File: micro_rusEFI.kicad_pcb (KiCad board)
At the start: 2 copper layers, 80.6 x 93.7 mm, 247 parts, among them CN1 100nF, CN2 100nF, CN3 100nF, CN4 100nF, J1 USB_B_Micro, J12 Conn_01x01, J13 Conn_01x01, J14 microSD_HC_Wuerth_693072010801, J15 Conn_01x01, J17 Conn_01x01, J19 Conn_01x06, J2 Conn_02x05_Odd_Even, J3 Conn_01x01, J4 Conn_02x05_Counter_Clockwise, J5 Conn_01x01, J7 TC2030, Q1 IPD30N06S2L-23, SW1 SW_Push, SW2 SW_Push, SW3 SW_Push, SW4 SW_Push, U1 STM32F427VGT6, U10 VNLD5090, U2 TLE8888QK, U3 molex_48pin_MRE, U31 MIC4427, U32 MIC4427, U33 MIC4427, U35 MCP6004, U36 MCP6004, U4 TLE9201SG, U46 MCP6004, U5 LM1117-3.3, U6 W25Q128JVSIQ, U7 XC6206 3.3V, U8 MCP6004, U9 VNLD5090, X1 8MHz 20pF, Y2 32768 Hz

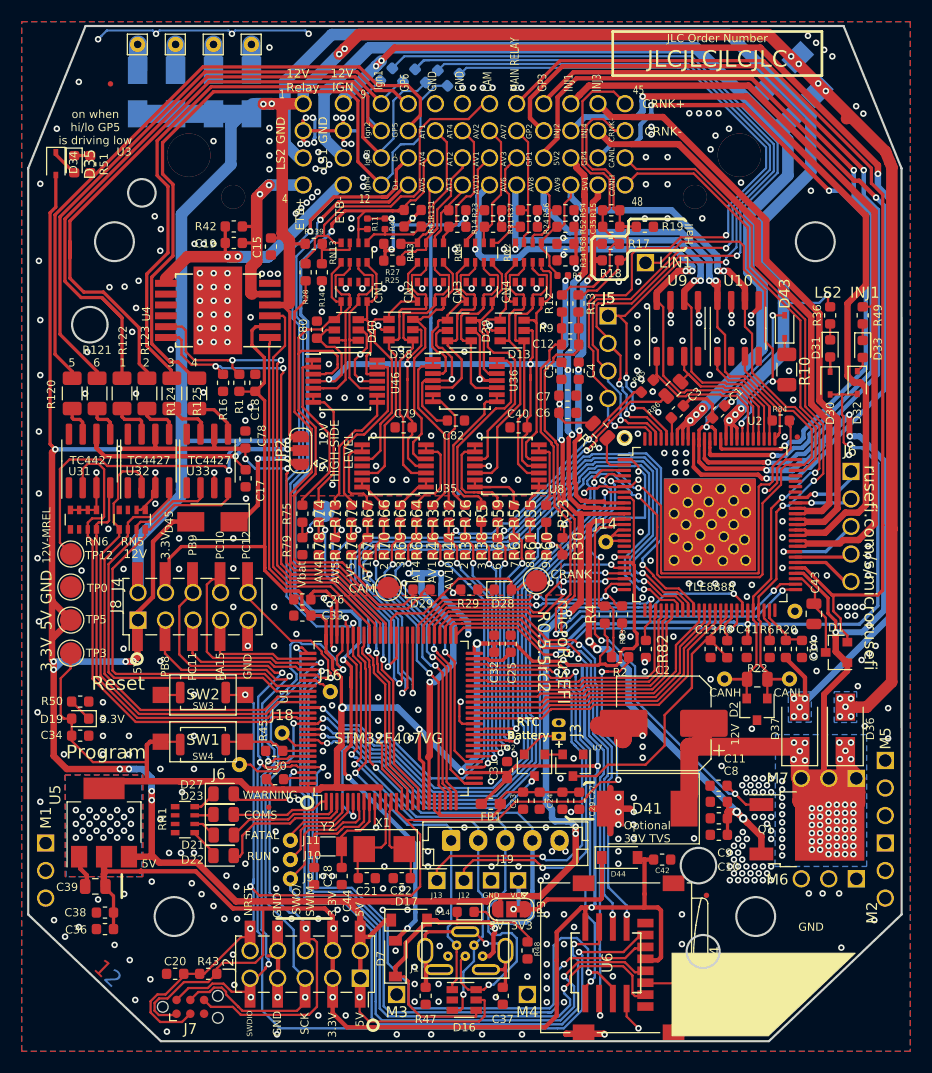
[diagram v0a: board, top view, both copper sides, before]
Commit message: Add files via upload
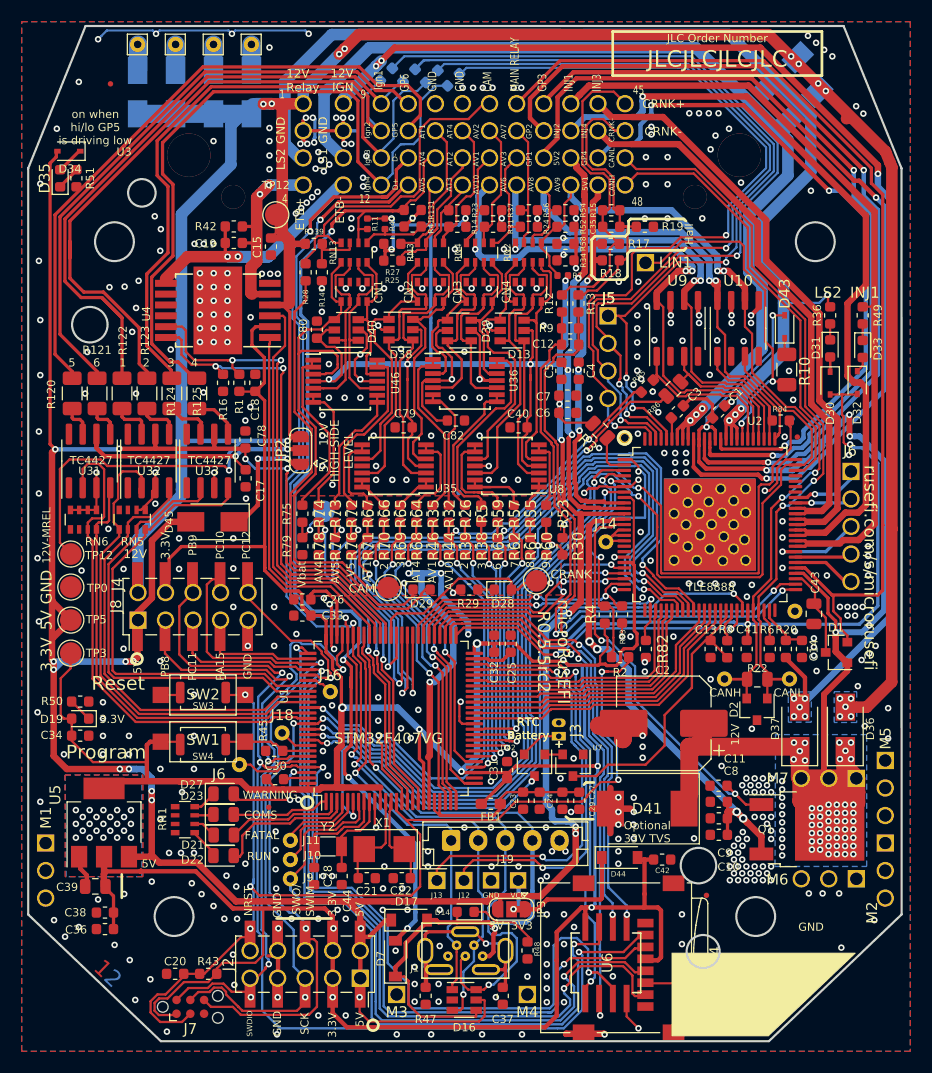
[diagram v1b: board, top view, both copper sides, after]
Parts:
- added TP12: 5V, TestPoint:TestPoint_Pad_D2.0mm, F.Cu at (43.5, 39.8)
- moved D35 1.84 mm to (23.6, 36.5), turned to 90 degrees
- moved R51 1.82 mm to (25.1, 36.5)
- moved D34 1.66 mm to (24.4, 34.0), turned to 180 degrees
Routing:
- net /12V_MREL: track 264.4 -> 266.7 mm
- net /5V: track 472.4 -> 473.8 mm
- net Net-(D35-Pad1): track 1.50 -> 2.20 mm

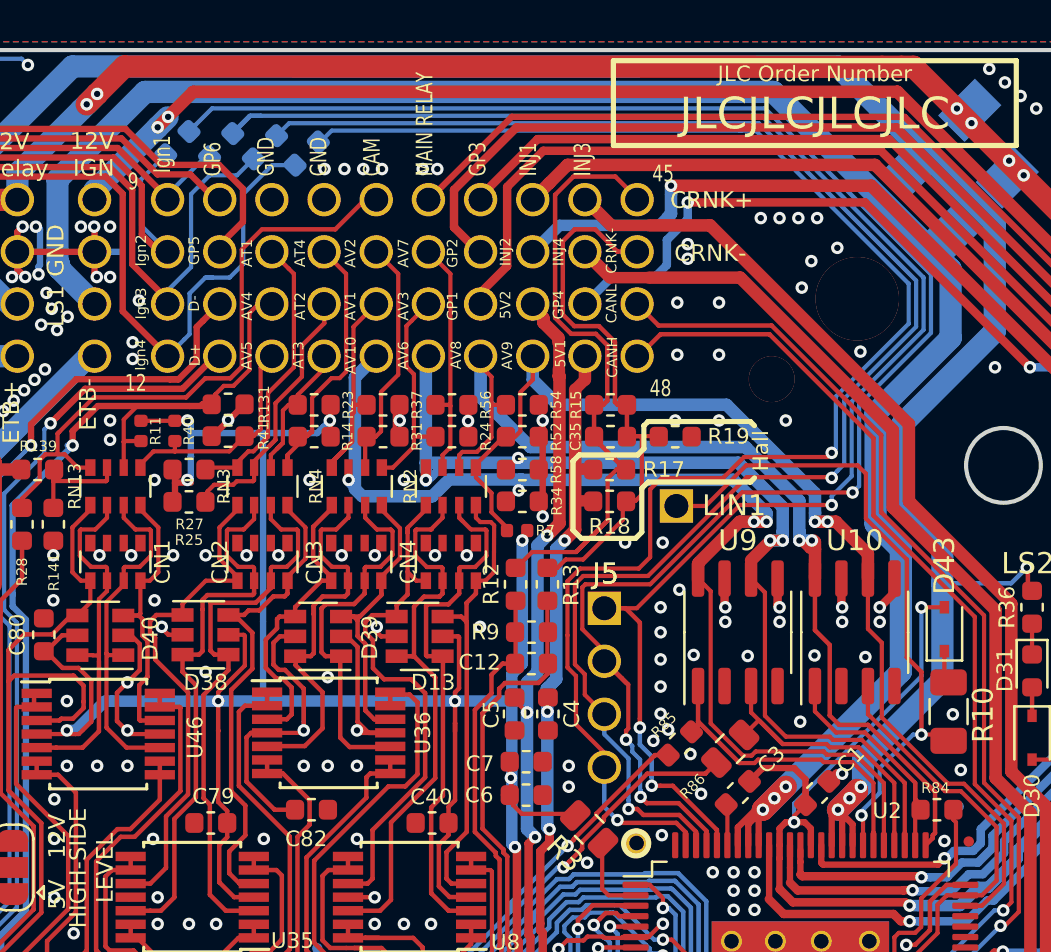
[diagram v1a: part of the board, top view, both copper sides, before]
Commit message: Add files via upload
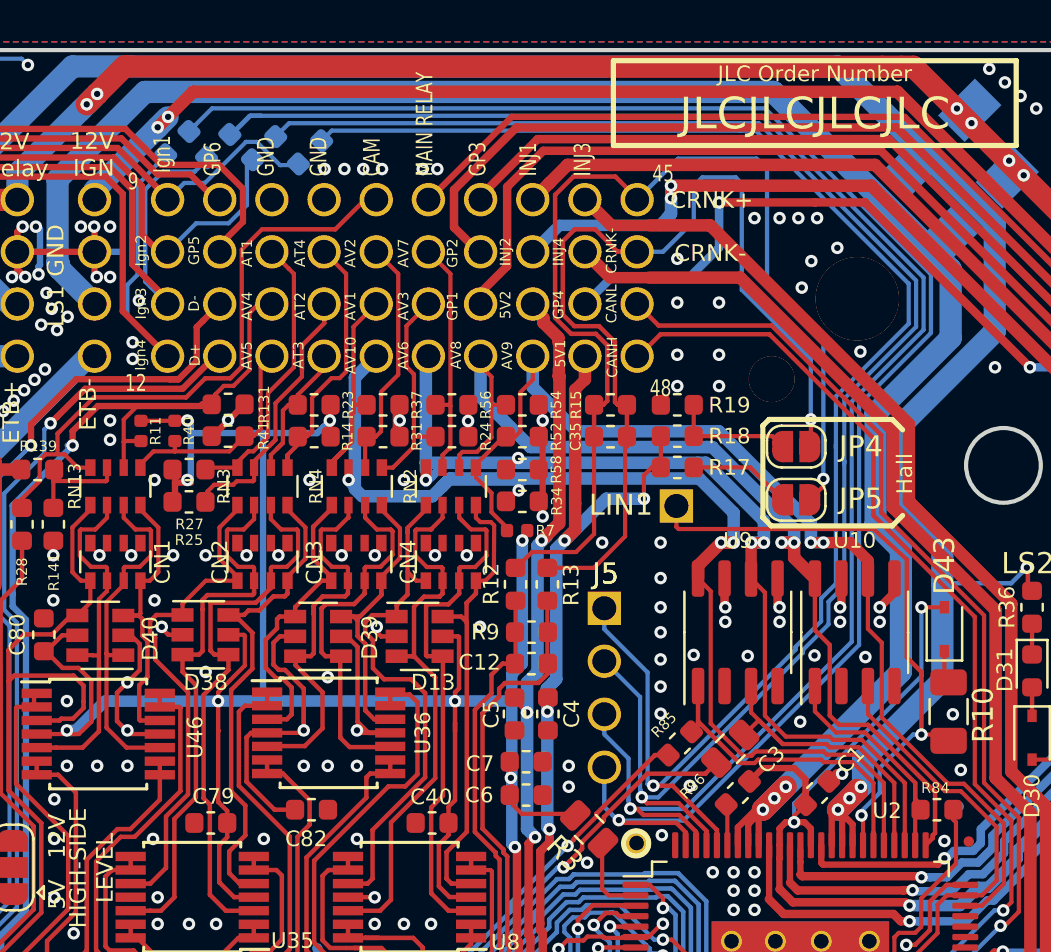
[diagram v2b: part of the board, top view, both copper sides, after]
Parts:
- added JP4: Jumper_NO_Small, Jumper:SolderJumper-2_P1.3mm_Open_RoundedPad1.0x1.5mm, F.Cu at (83.3, 41.4)
- added JP5: SolderJumper-2_P1.3mm_Open_RoundedPad1.0x1.5mm, Jumper:SolderJumper-2_P1.3mm_Open_RoundedPad1.0x1.5mm, F.Cu at (83.3, 44.0)
- R17: value DNP -> 2.2k
- R18, R19: value DNP -> 4.7K
- moved R81 6.22 mm to (53.6, 26.9)
- moved R18 4.50 mm to (77.6, 40.9)
- moved R21 4.27 mm to (60.0, 27.3)
- moved R33 4.16 mm to (57.8, 27.1)
- moved R17 3.24 mm to (77.6, 42.4)
- moved R80 2.24 mm to (55.6, 27.0)
- moved R19 1.53 mm to (77.6, 39.4), turned to 0 degrees
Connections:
- R17 pad 2: /CRNK+ -> Net-(JP5-Pad2)
- R18 pad 2: /CRNK- -> Net-(JP4-Pad2)
- R19 pad 2: /CRNK- -> Net-(JP4-Pad2)
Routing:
- net /CRNK+: track 31.2 -> 52.2 mm, vias 0 -> 1
- net /CRNK-: track 27.4 -> 47.1 mm, vias 0 -> 1
- net /5V1: track 37.9 -> 44.4 mm, vias 3 -> 4
- net /TLE8888-1QK/IGN_OUT_2: track 83.6 -> 77.1 mm, vias 3 -> 1
- net /TLE8888-1QK/IGN_OUT_4: track 74.9 -> 81.2 mm, vias 2 -> 1
- net Net-(JP4-Pad2): track 0.00 -> 5.92 mm
- net /Ign1: track 59.7 -> 64.6 mm
- net /TLE8888-1QK/IGN_OUT_3: track 75.6 -> 80.6 mm, vias 2 -> 1
- net Net-(JP5-Pad2): track 0.00 -> 4.90 mm
- net /TLE8888-1QK/IGN_OUT_1: track 78.8 -> 75.6 mm, vias 3 -> 1
- net /LINBUS: track 31.8 -> 29.5 mm
- net /Ign4: track 68.5 -> 66.3 mm
- net /AV10: track 56.9 -> 58.7 mm
- net /AV6: track 50.2 -> 48.5 mm
- net /Ign2: track 62.7 -> 64.1 mm
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
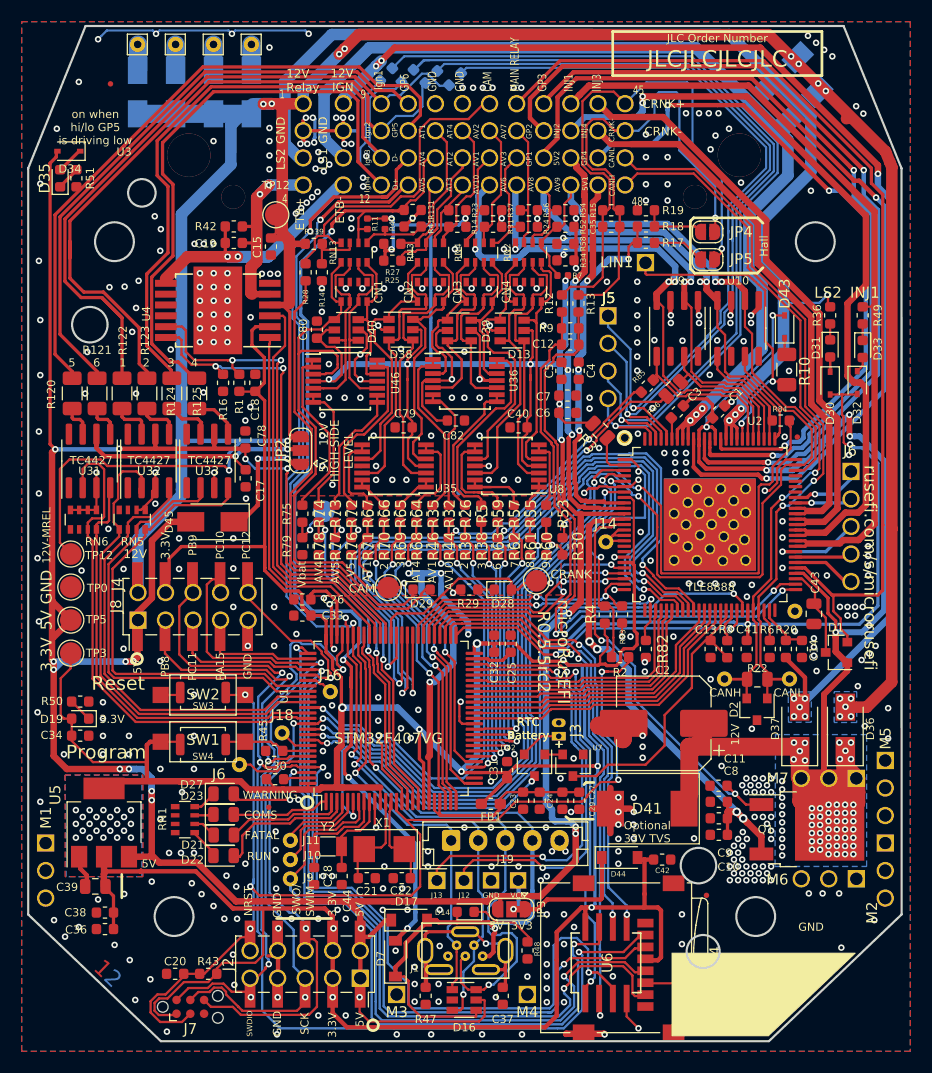
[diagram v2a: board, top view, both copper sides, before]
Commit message: Add files via upload
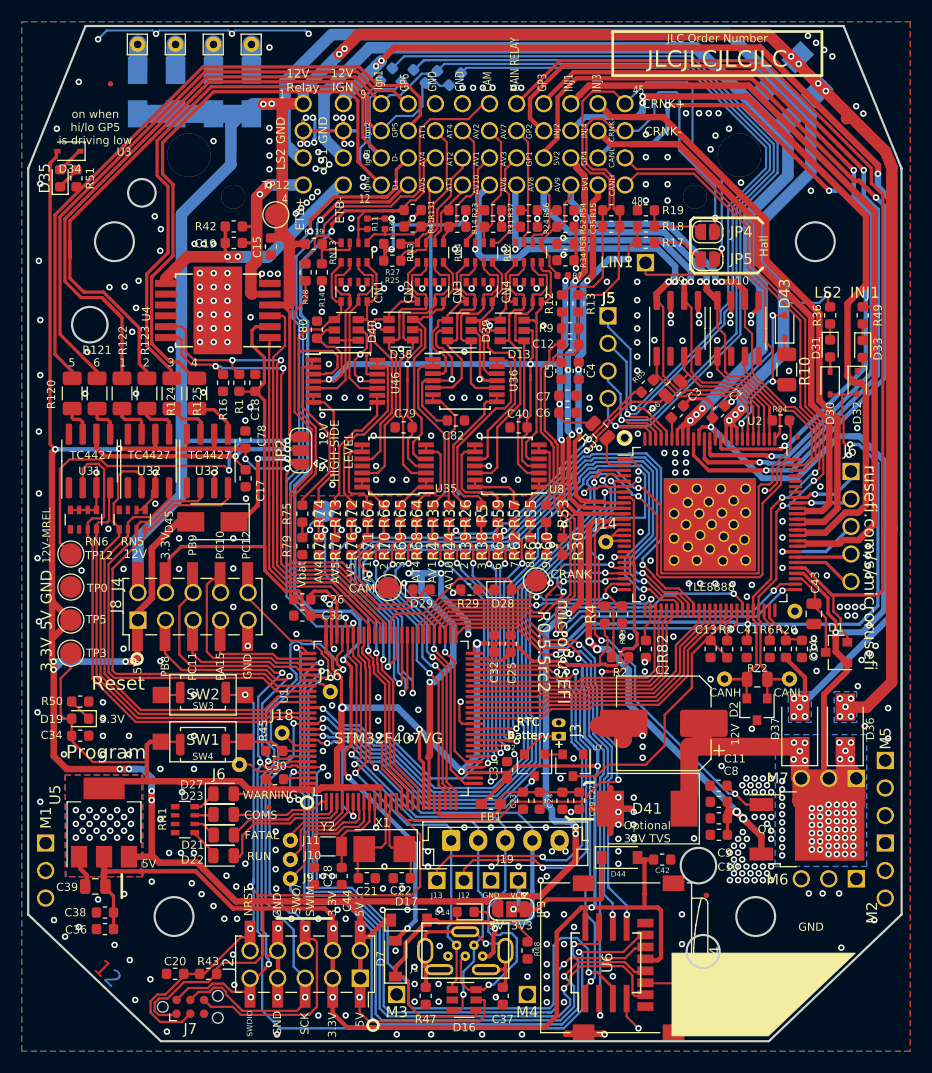
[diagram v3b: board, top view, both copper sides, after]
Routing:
- net /12V_SAFE: track 138.0 -> 134.3 mm, vias 57 -> 54
- net /GP1: track 83.1 -> 81.1 mm
- net /GP2: track 80.5 -> 81.9 mm
- net /5V: track 473.8 -> 474.5 mm
- net GND: vias 470 -> 472
